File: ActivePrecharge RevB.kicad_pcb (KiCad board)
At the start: 2 copper layers, 59 parts, among them IC1 AMC1350DWVR, IC2 AMC1350DWVR, U1 LT1963AEST-3.3_TRPBF, U2 TLV9001IDBVR, U3 TLV9001IDBVR

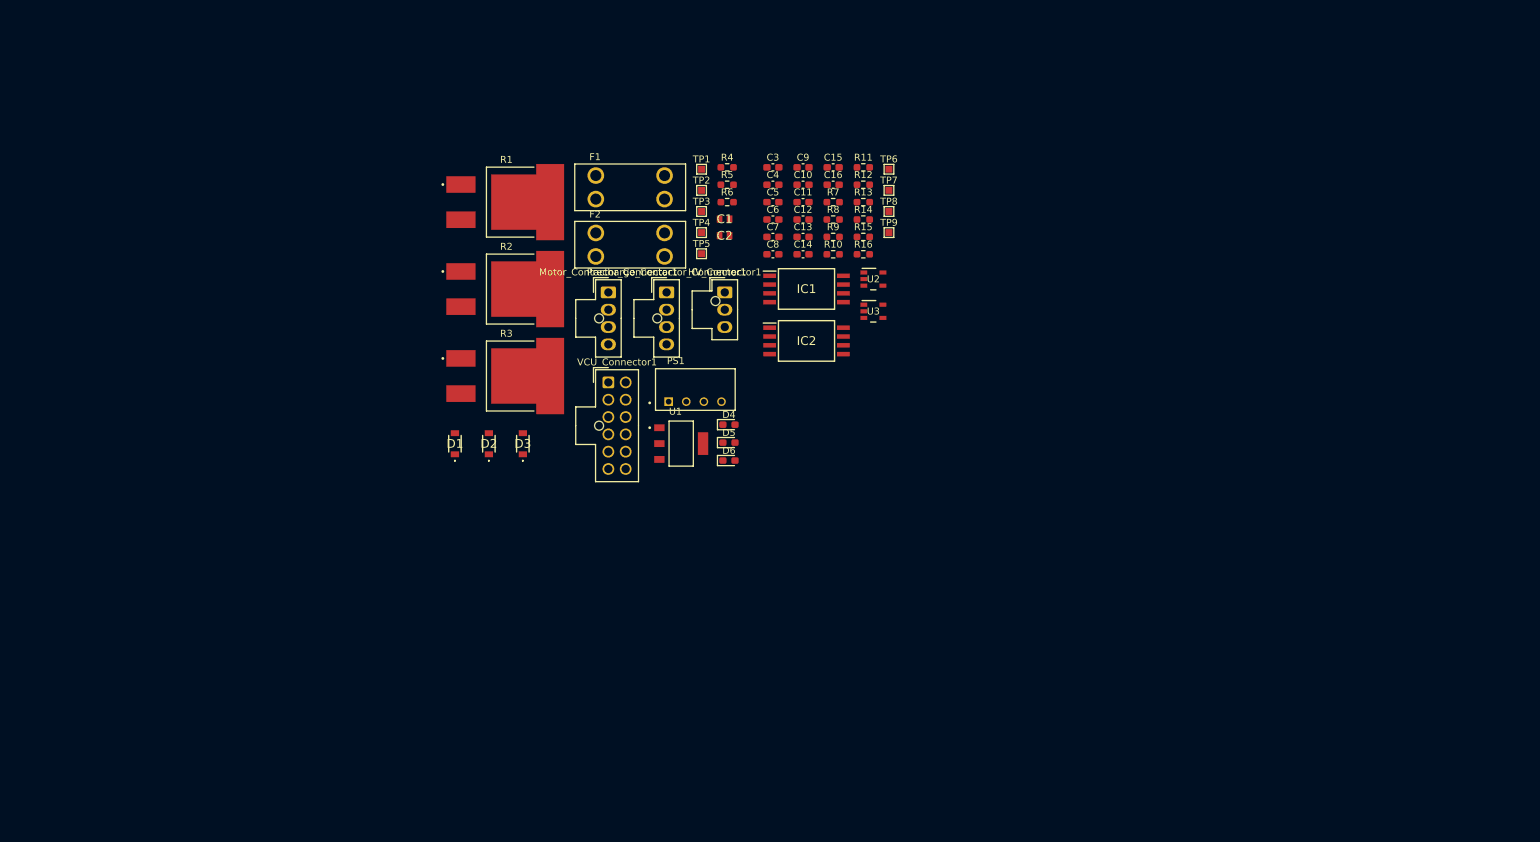
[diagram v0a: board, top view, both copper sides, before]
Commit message: First Initial PCB Layout Finished
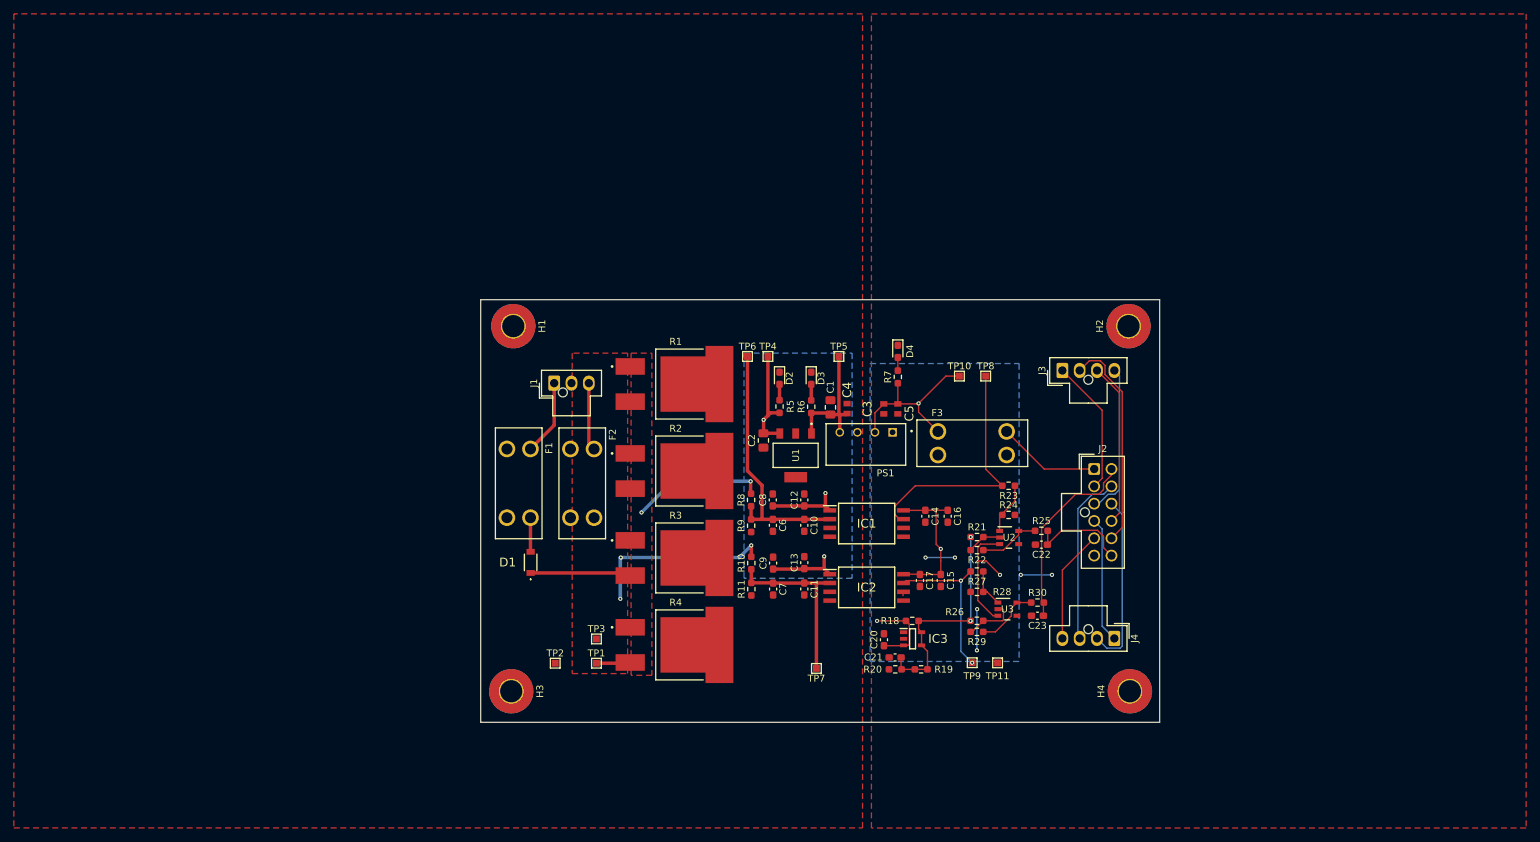
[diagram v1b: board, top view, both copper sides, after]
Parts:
- removed D5, D6: LED, LED_SMD:LED_0603_1608Metric_Pad1.05x0.95mm_HandSolder
- removed HV_Connector1: Conn_01x03, Connector_Molex:Molex_Nano-Fit_105309-xx03_1x03_P2.50mm_Vertical
- removed Motor_Contactor_Connector1, Precharge_Contactor_Connector1: Conn_01x04, Connector_Molex:Molex_Nano-Fit_105309-xx04_1x04_P2.50mm_Vertical
- removed R12, R14: 10k, Resistor_SMD:R_0603_1608Metric_Pad0.98x0.95mm_HandSolder
- removed R13: 15k, Resistor_SMD:R_0603_1608Metric_Pad0.98x0.95mm_HandSolder
- removed R15, R16: 10, Resistor_SMD:R_0603_1608Metric_Pad0.98x0.95mm_HandSolder
- removed VCU_Connector1: Conn_02x06_Counter_Clockwise, Connector_Molex:Molex_Nano-Fit_105310-xx12_2x06_P2.50mm_Vertical
- added C17: 100nF, Capacitor_SMD:C_0603_1608Metric_Pad1.08x0.95mm_HandSolder, F.Cu at (162.7, 100.3)
- added C20: 0.1uF, Capacitor_SMD:C_0603_1608Metric_Pad1.08x0.95mm_HandSolder, F.Cu at (157.5, 108.9)
- added C21: 0.47uF, Capacitor_SMD:C_0603_1608Metric_Pad1.08x0.95mm_HandSolder, F.Cu at (159.1, 111.4)
- added C22: 10nF, Capacitor_SMD:C_0603_1608Metric_Pad1.08x0.95mm_HandSolder, F.Cu at (180.2, 95.1)
- added C23: 10nF, Capacitor_SMD:C_0603_1608Metric_Pad1.08x0.95mm_HandSolder, F.Cu at (179.7, 105.4)
- added F3: 15A, ActivePrecharge-RevB:FUSE_3568, F.Cu at (170.2, 80.5)
- added H1: MountingHole_Pad, MountingHole:MountingHole_3.2mm_M3_Pad_TopBottom, F.Cu at (104.0, 63.6)
- added H2: MountingHole_Pad, MountingHole:MountingHole_3.2mm_M3_Pad_TopBottom, F.Cu at (192.8, 63.6)
- added H3: MountingHole_Pad, MountingHole:MountingHole_3.2mm_M3_Pad_TopBottom, F.Cu at (103.7, 116.3)
- added H4: MountingHole_Pad, MountingHole:MountingHole_3.2mm_M3_Pad_TopBottom, F.Cu at (193.0, 116.3)
- added IC3: ZXRE160AET5TA, ActivePrecharge-RevB:SOT95P280X100-5N, F.Cu at (161.6, 108.7)
- added J1: HVConnector, Connector_Molex:Molex_Nano-Fit_105309-xx03_1x03_P2.50mm_Vertical, F.Cu at (109.9, 71.8)
- added J2: ExportConnector, Connector_Molex:Molex_Nano-Fit_105310-xx12_2x06_P2.50mm_Vertical, F.Cu at (187.8, 84.2)
- added J3: PrechargeContactor, Connector_Molex:Molex_Nano-Fit_105309-xx04_1x04_P2.50mm_Vertical, F.Cu at (183.2, 70.0)
- added J4: MainContactor, Connector_Molex:Molex_Nano-Fit_105309-xx04_1x04_P2.50mm_Vertical, F.Cu at (190.8, 108.7)
- added R18: 1k, Resistor_SMD:R_0603_1608Metric_Pad0.98x0.95mm_HandSolder, F.Cu at (161.6, 106.1)
- added R19: 5.1k, Resistor_SMD:R_0603_1608Metric_Pad0.98x0.95mm_HandSolder, F.Cu at (162.9, 113.1)
- added R20: 15k, Resistor_SMD:R_0603_1608Metric_Pad0.98x0.95mm_HandSolder, F.Cu at (159.1, 113.1)
- added R21: 2.49k, Resistor_SMD:R_0603_1608Metric_Pad0.98x0.95mm_HandSolder, F.Cu at (170.9, 94.0)
- added R22: 15k, Resistor_SMD:R_0603_1608Metric_Pad0.98x0.95mm_HandSolder, F.Cu at (170.9, 95.9)
- added R23: 2.49k, Resistor_SMD:R_0603_1608Metric_Pad0.98x0.95mm_HandSolder, F.Cu at (175.5, 86.6)
- added R24: 15k, Resistor_SMD:R_0603_1608Metric_Pad0.98x0.95mm_HandSolder, F.Cu at (175.5, 90.8)
- added R25: 10, Resistor_SMD:R_0603_1608Metric_Pad0.98x0.95mm_HandSolder, F.Cu at (180.2, 93.1)
- added R26: 2.49k, Resistor_SMD:R_0603_1608Metric_Pad0.98x0.95mm_HandSolder, F.Cu at (170.9, 106.1)
- added R27: 2.49k, Resistor_SMD:R_0603_1608Metric_Pad0.98x0.95mm_HandSolder, F.Cu at (170.9, 99.0)
- added R28: 15k, Resistor_SMD:R_0603_1608Metric_Pad0.98x0.95mm_HandSolder, F.Cu at (170.9, 102.0)
- added R29: 15k, Resistor_SMD:R_0603_1608Metric_Pad0.98x0.95mm_HandSolder, F.Cu at (170.9, 107.7)
- added R30: 10, Resistor_SMD:R_0603_1608Metric_Pad0.98x0.95mm_HandSolder, F.Cu at (179.7, 103.5)
- added TP10: 3V3, TestPoint:TestPoint_Pad_1.0x1.0mm, F.Cu at (168.4, 70.8)
- added TP11: LVGND, TestPoint:TestPoint_Pad_1.0x1.0mm, F.Cu at (173.9, 112.2)
- C1, C2: footprint ActivePrecharge-RevB:CAPC1709X100N -> Capacitor_SMD:C_0805_2012Metric_Pad1.18x1.45mm_HandSolder
- C10, C11: value 1uF -> 1nF
- C13, C14, C6: value 100nF -> 1uF
- C15: value 10nF -> 1uF
- C16: value 10nF -> 100nF
- C3, C4: footprint Capacitor_SMD:C_0603_1608Metric_Pad1.08x0.95mm_HandSolder -> ActivePrecharge-RevB:CAPC1709X100N
- C5: value 100nF -> 1uF; footprint Capacitor_SMD:C_0603_1608Metric_Pad1.08x0.95mm_HandSolder -> ActivePrecharge-RevB:CAPC1709X100N
- C7: value 1nF -> 1uF
- C8: value 1nF -> 100nF
- C9: value 1uF -> 100nF
- D2, D3: value RSX068MP2STR -> LED; footprint ActivePrecharge-RevB:RSX068MP2STR -> LED_SMD:LED_0603_1608Metric_Pad1.05x0.95mm_HandSolder
- F1, F2: value Fuse -> 15A
- R10, R8: value 2.49k -> 100k
- R11: value 15k -> 2.49k
- R4: value 120 -> 330; footprint Resistor_SMD:R_0603_1608Metric_Pad0.98x0.95mm_HandSolder -> ActivePrecharge-RevB:RES_PWR263S-35-3300F
- R5: value 768 -> 1k
- R6: value 120 -> 1k
- R7: value 100k -> 1k
- R9: value 100k -> 2.49k
- U1: value LT1963AEST-3.3_TRPBF -> LT1963AEST-3.3#TRPBF
- moved TP1 72.9 mm to (116.0, 112.2)
- moved TP2 71.4 mm to (110.0, 112.2)
- moved TP7 69.8 mm to (147.8, 113.0), turned to 180 degrees
- moved R4 69.3 mm to (127.3, 109.6)
- moved TP3 63.5 mm to (116.0, 108.8)
- moved TP9 63.2 mm to (170.2, 112.2)
- moved R11 63.0 mm to (138.4, 101.6), turned to 90 degrees
- moved C15 61.6 mm to (165.7, 100.3), turned to -90 degrees
- moved C9 57.3 mm to (141.5, 97.8), turned to 90 degrees
- moved C11 55.8 mm to (146.0, 101.5), turned to -90 degrees
- moved C7 50.8 mm to (141.5, 101.5), turned to -90 degrees
- moved C16 50.6 mm to (166.7, 91.0), turned to -90 degrees
- moved C10 49.2 mm to (146.0, 92.4), turned to -90 degrees
- moved U3 47.1 mm to (175.3, 104.5)
- moved C13 47.0 mm to (146.0, 97.7), turned to 90 degrees
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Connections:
- C10 pad 1: REG_3V3 -> /Voltage_Sense/Vin1
- C11 pad 1: 3V3 -> /Voltage_Sense/Vin2
- C11 pad 2: LVGND -> HVGND
- C12 pad 1: 3V3 -> REG_3V3
- C12 pad 2: LVGND -> HVGND
- C13 pad 1: 3V3 -> REG_3V3
- C13 pad 2: LVGND -> HVGND
- C15 pad 1: /VOut1 -> 3V3
- C16 pad 1: /VOut2 -> 3V3
- C3 pad 1: /Voltage_Sense/Vin1 -> 3V3
- C3 pad 2: HVGND -> LVGND
- C4 pad 1: /Voltage_Sense/Vin2 -> HVGND
- C4 pad 2: HVGND -> ISO_5V
- C5 pad 1: REG_3V3 -> 3V3
- C5 pad 2: HVGND -> LVGND
- C6 pad 1: REG_3V3 -> /Voltage_Sense/Vin1
- C7 pad 1: /Voltage_Sense/Vin1 -> /Voltage_Sense/Vin2
- C8 pad 1: /Voltage_Sense/Vin2 -> REG_3V3
- D2 pad 1: Net-(D2-K) -> HVGND
- D2 pad 2: HVGND -> Net-(D2-A)
- D3 pad 1: HV- -> HVGND
- F2 pad 2: Net-(D3-A) -> HV-
- R10 pad 1: HVGND -> /Voltage_Sense/Vin2
- R10 pad 2: /Voltage_Sense/Vin2 -> HV-
- R11 pad 1: Net-(U2-OUT) -> HVGND
- R11 pad 2: Net-(U2-IN-) -> /Voltage_Sense/Vin2
- R4 pad 1: REG_3V3 -> HV-
- R4 pad 2: Net-(D4-A) -> HV+
- R5 pad 1: ISO_5V -> REG_3V3
- R5 pad 2: Net-(D5-A) -> Net-(D2-A)
- R6 pad 1: 3V3 -> ISO_5V
- R6 pad 2: Net-(D6-A) -> Net-(D3-A)
- R7 pad 1: /Voltage_Sense/Vin1 -> 3V3
- R7 pad 2: HV+ -> Net-(D4-A)
- R8 pad 1: HVGND -> /Voltage_Sense/Vin1
- R8 pad 2: /Voltage_Sense/Vin1 -> HV+
- R9 pad 1: /Voltage_Sense/Vin2 -> HVGND
- R9 pad 2: HV- -> /Voltage_Sense/Vin1
- U1 pad 4: HVGND -> (no net)
- U2 pad 1: Net-(U2-OUT) -> Net-(U2-+)
- U2 pad 2: LVGND -> Net-(U2--)
- U2 pad 3: /Voltage_Sense/V1 -> 3V3
- U2 pad 4: Net-(U2-IN-) -> LVGND
- U2 pad 5: 3V3 -> Net-(R22-Pad1)
- U3 pad 2: LVGND -> Net-(U3--)
- U3 pad 3: /Voltage_Sense/V2 -> 3V3
- U3 pad 4: Net-(U3-IN-) -> LVGND
- U3 pad 5: 3V3 -> Net-(R29-Pad1)
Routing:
- net 3V3: track 0.00 -> 77.1 mm, vias 0 -> 4
- net HV+: track 0.00 -> 38.9 mm, vias 0 -> 2
- net /Voltage_Sense/Vin1: track 0.00 -> 37.6 mm
- net REG_3V3: track 0.00 -> 36.6 mm, vias 0 -> 3
- net /Voltage_Sense/V1: track 0.00 -> 36.3 mm
- net REG_0V8: track 0.00 -> 32.6 mm, vias 0 -> 2
- net /Pre-: track 0.00 -> 31.1 mm
- net HV-: track 0.00 -> 28.1 mm, vias 0 -> 3
- net /VOut2: track 0.00 -> 27.5 mm
- net /Voltage_Sense/Vin2: track 0.00 -> 25.6 mm
- net /Motor-: track 0.00 -> 25.5 mm
- net /MotorSense-: track 0.00 -> 25.0 mm
- net /PreSense-: track 0.00 -> 23.5 mm
- net /Voltage_Sense/V2: track 0.00 -> 22.9 mm, vias 0 -> 2
- net /PreSense+: track 0.00 -> 22.0 mm
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- added copper zone on B.Cu, net 3V3
- added copper zone on F.Cu, net HV+
- added copper zone on F.Cu, net HV-
- added copper zone on F.Cu, net HVGND
- added copper zone on F.Cu, net LVGND
- added copper zone on B.Cu, net REG_3V3
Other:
- board outline added: 98 x 61 mm
